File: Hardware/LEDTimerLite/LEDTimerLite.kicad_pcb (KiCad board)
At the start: 4 copper layers, 37.3 x 23.1 mm, 27 parts, among them J1 Program, J2 LED, J3 PWR, Q1 S8050, SW1 SW_Push, SW4 SW_PWR, U1 AP7383-36WW7, U2 PIC16LF18326, U4 BCR_421U_E6327, Y1 32.768 kHz

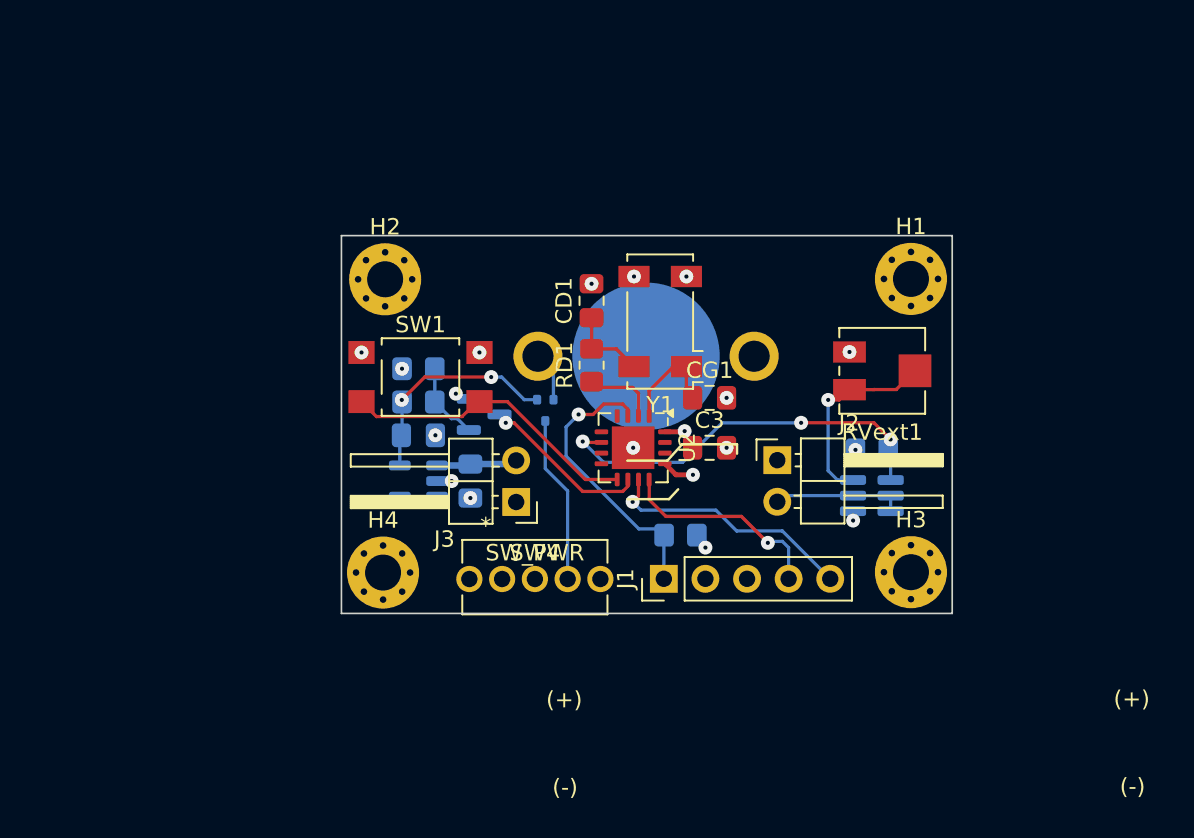
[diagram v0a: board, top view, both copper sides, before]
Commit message: LTL: try new PCB layout
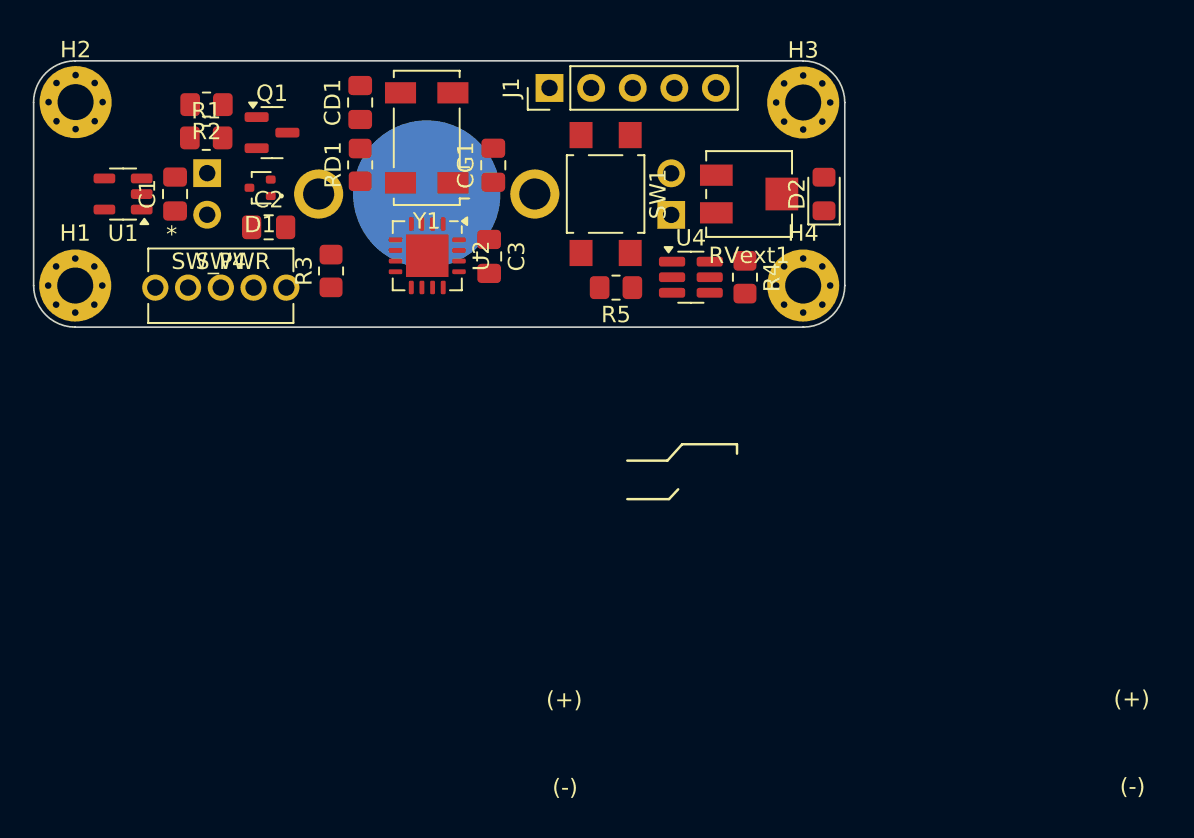
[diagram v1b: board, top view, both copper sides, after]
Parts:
- added D2: Red LED, LED_SMD:LED_0805_2012Metric_Pad1.15x1.40mm_HandSolder, F.Cu at (138.8, 64.8)
- added R4: 560, Resistor_SMD:R_0805_2012Metric_Pad1.20x1.40mm_HandSolder, F.Cu at (134.0, 69.8)
- C1, C2, D1, Q1, R1, R2, R3, R5, U1, U4: moved to F.Cu
- J2, J3: moved to B.Cu
- moved H1 51.0 mm to (93.1, 70.4)
- moved H4 31.1 mm to (137.5, 70.4)
- moved J1 30.8 mm to (122.1, 58.3)
- moved H3 29.4 mm to (137.5, 59.2)
- moved J3 27.6 mm to (101.1, 63.5)
- moved R3 26.7 mm to (108.7, 69.5), turned to 90 degrees
- moved SW4 26.2 mm to (100.0, 70.5)
- moved C1 25.1 mm to (99.2, 64.8), turned to 90 degrees
- moved U1 25.1 mm to (96.0, 64.8)
- moved D1 22.1 mm to (104.4, 64.4), turned to 180 degrees
- moved H2 21.8 mm to (93.1, 59.2)
- moved Q1 21.5 mm to (105.1, 61.0)
- moved R1 20.7 mm to (101.1, 61.3)
- moved R2 20.7 mm to (101.1, 59.3)
- moved CG1 19.4 mm to (118.6, 63.0), turned to 90 degrees
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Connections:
- U2 pad 8: unconnected-(U2-RC1-Pad8) -> /LED
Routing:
- net /LED_EN_PWM: track 24.5 -> 0.00 mm, vias 3 -> 0
- net +5V: track 24.5 -> 0.00 mm
- net Net-(U2-RC0): track 18.3 -> 0.00 mm
- net /~{MCLR}/VPP: track 17.6 -> 0.00 mm, vias 1 -> 0
- net /ICSPCLK_RXD: track 15.5 -> 0.00 mm, vias 1 -> 0
- net Net-(U1-VOUT): track 13.3 -> 0.00 mm, vias 2 -> 0
- net /ICSPDAT_TXD: track 12.9 -> 0.00 mm, vias 1 -> 0
- net Net-(U4-Rext): track 12.1 -> 0.00 mm, vias 1 -> 0
- net /LDO_SENSE: track 10.4 -> 0.00 mm, vias 1 -> 0
- net Net-(SW4-C): track 10.2 -> 0.00 mm
- net Net-(J2-Pin_2): track 8.03 -> 0.00 mm
- net Net-(U2-RA5): track 6.34 -> 0.00 mm
- net Net-(CD1-Pad1): track 4.94 -> 0.00 mm
- net Net-(Q1-B): track 4.82 -> 0.00 mm
- net Net-(U2-RA4): track 4.55 -> 0.00 mm
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- removed copper zone on In2.Cu, net +3V3
- removed copper zone on In1.Cu, net GND
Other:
- board size 37.3 x 23.1 mm -> 49.5 x 16.3 mm
